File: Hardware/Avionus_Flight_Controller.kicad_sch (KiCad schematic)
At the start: 0 parts

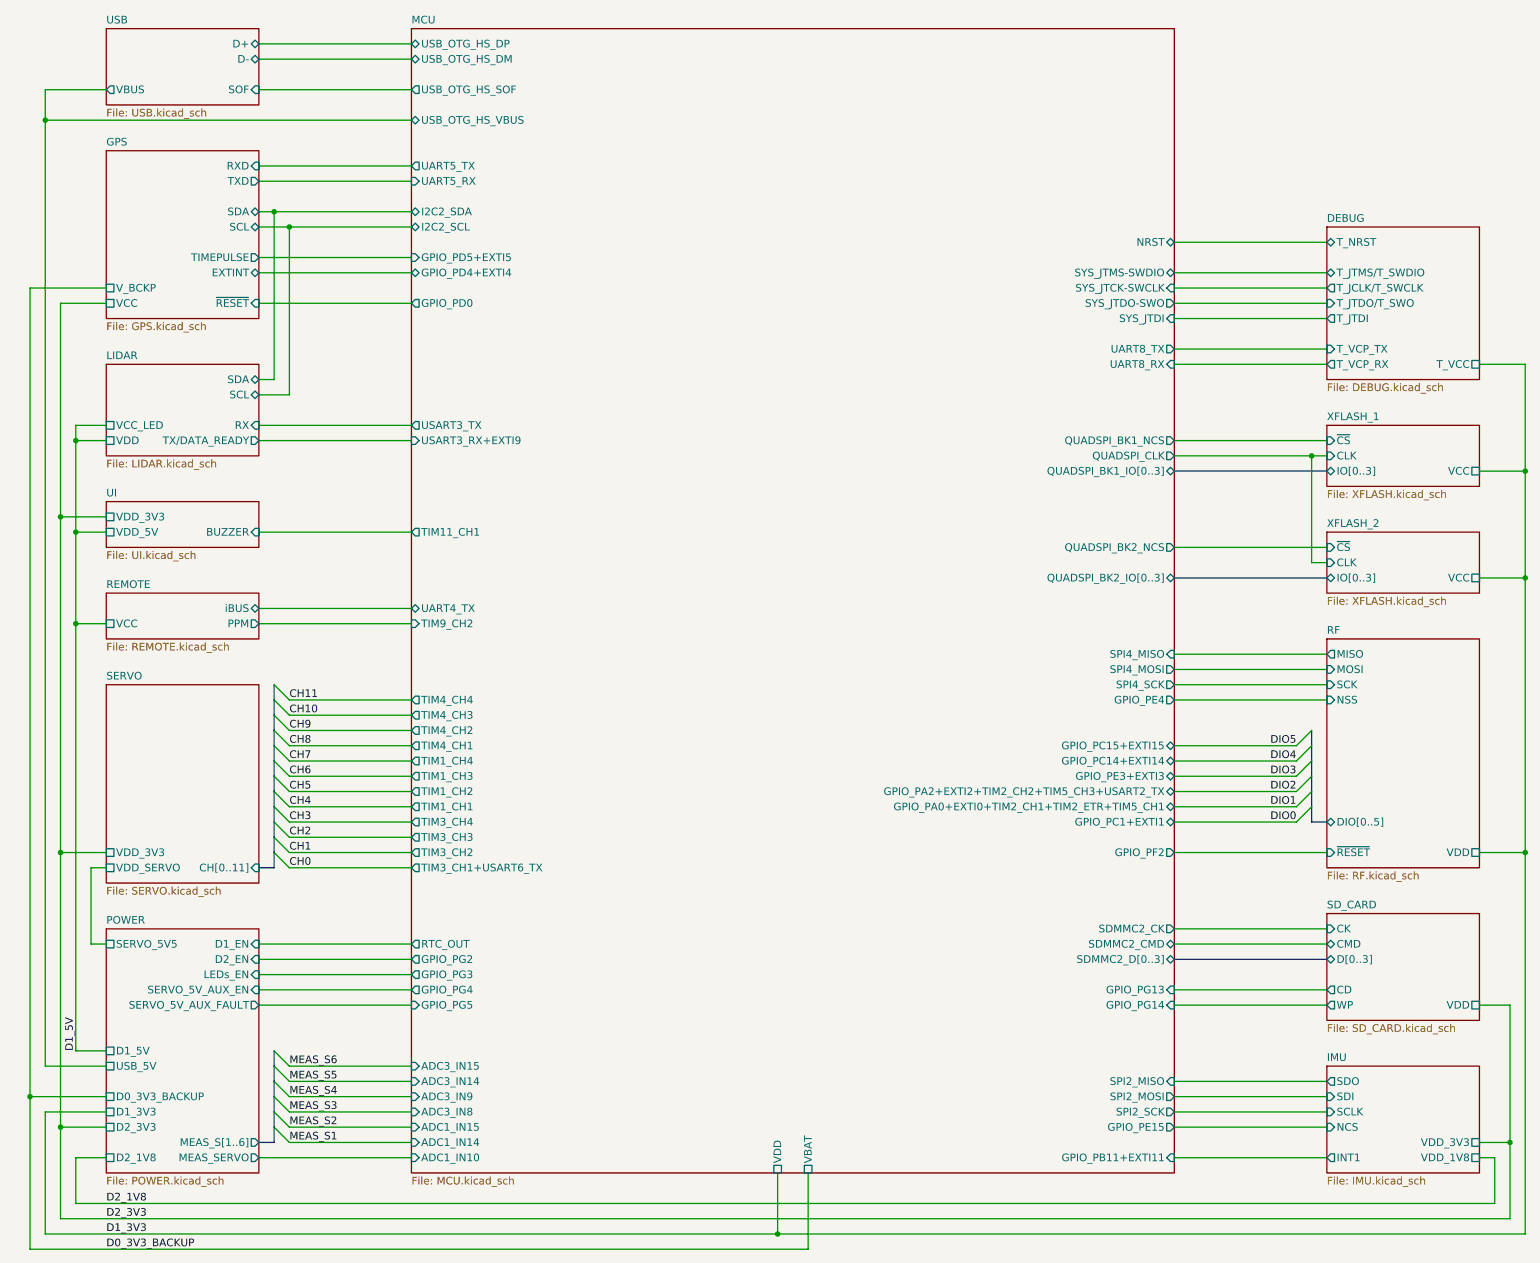
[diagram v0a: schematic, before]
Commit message: Checkpoint
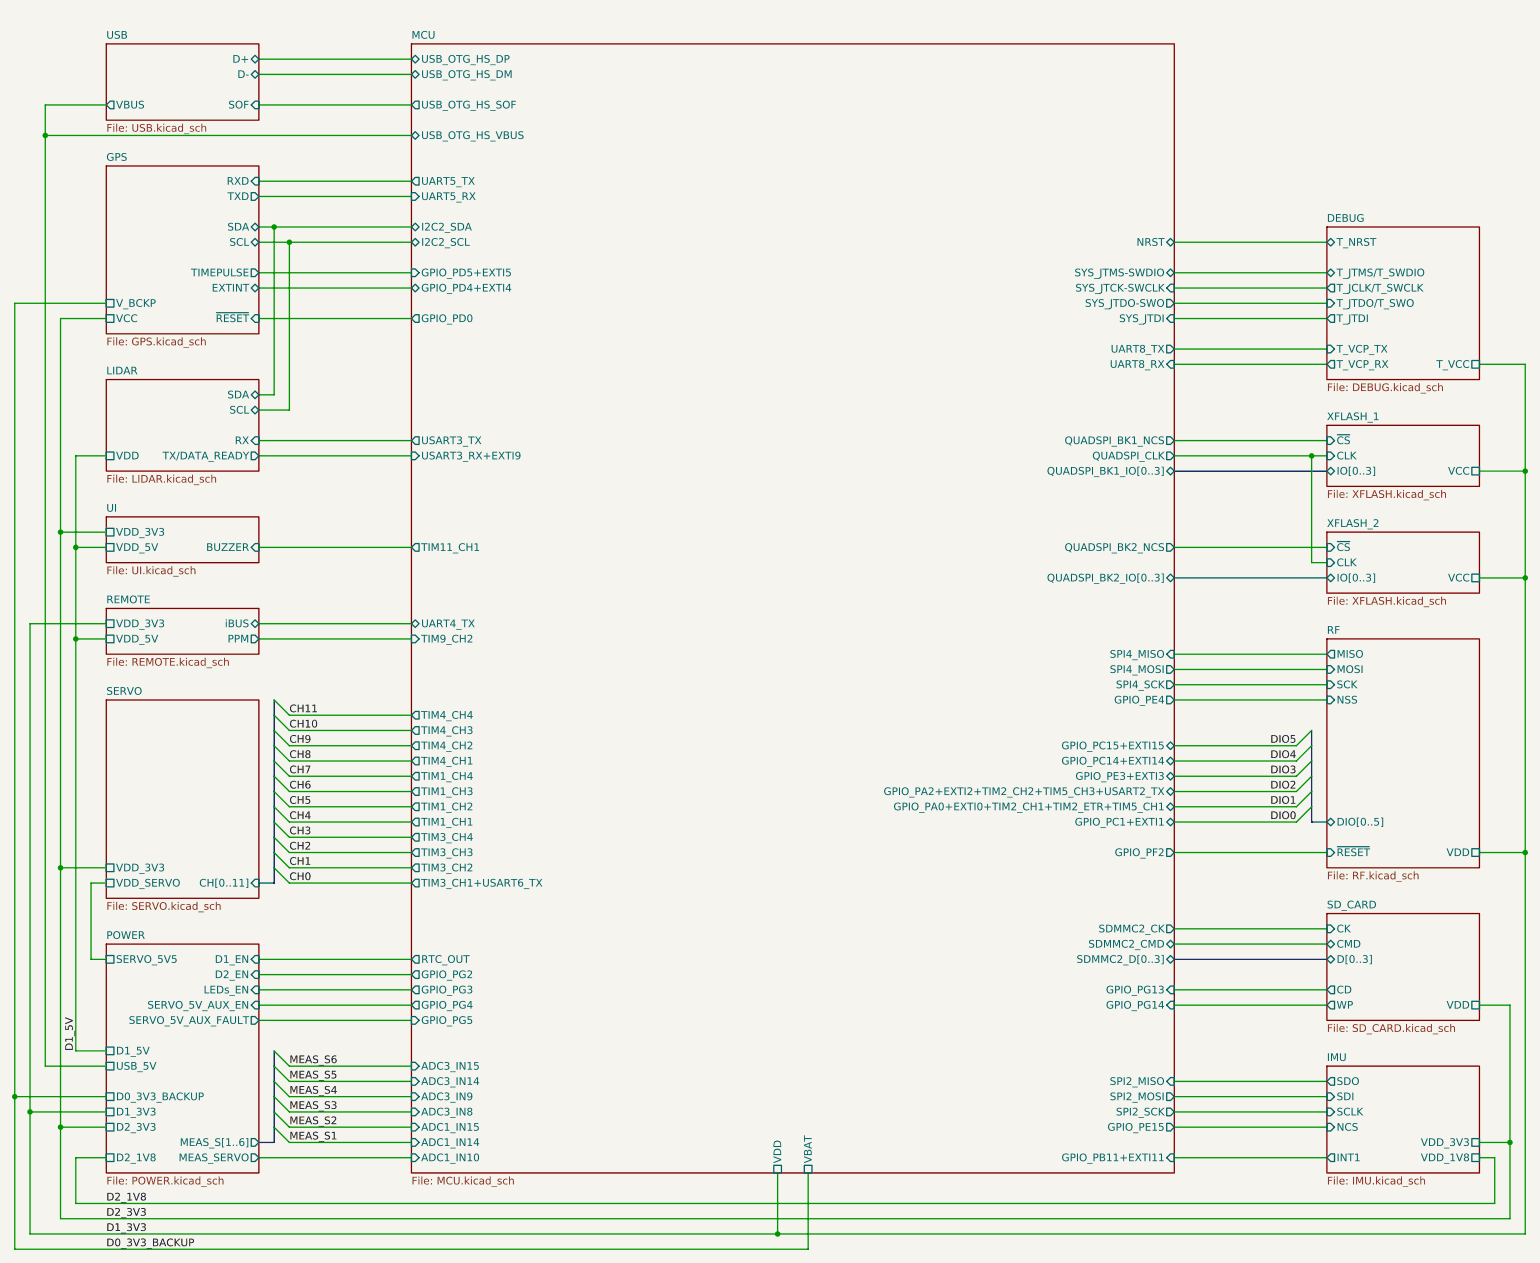
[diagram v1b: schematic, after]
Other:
- sheet LIDAR ports: added none; removed VCC_LED
- sheet REMOTE ports: added VDD_3V3, VDD_5V; removed VCC
